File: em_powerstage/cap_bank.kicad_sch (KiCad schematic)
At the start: 20 parts

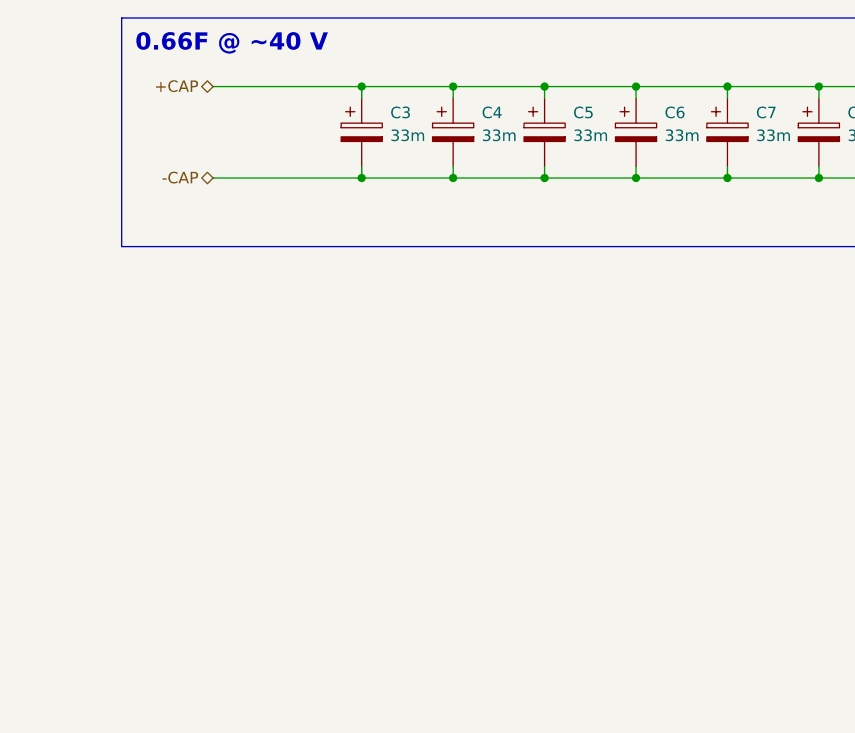
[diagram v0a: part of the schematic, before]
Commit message: updated power stage board
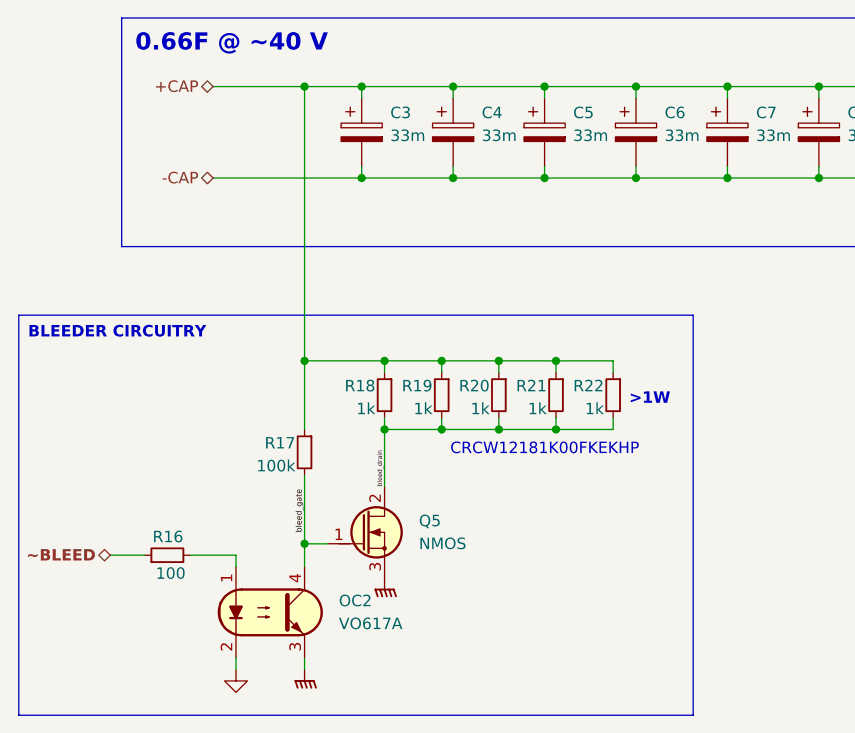
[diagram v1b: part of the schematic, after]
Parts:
- added OC2: VO617A, PCM_Package_DIP_AKL:DIP-4_W7.62mm_LongPads, symbol PCM_Optocoupler_AKL:VO617A
- added Q5: NMOS, Package_TO_SOT_SMD:SOT-23-3, symbol PCM_Transistor_MOSFET_AKL:Q_NMOS-D_Generic_GDS
- added R16: 100, Resistor_SMD:R_0805_2012Metric_Pad1.20x1.40mm_HandSolder, symbol Device:R_Small
- added R17: 100k, Resistor_SMD:R_0805_2012Metric_Pad1.20x1.40mm_HandSolder, symbol Device:R_Small
- added R18, R19, R20, R21, R22: 1k, Resistor_SMD:R_1218_3246Metric_Pad1.22x4.75mm_HandSolder, symbol Device:R_Small
- C10, C11, C12, C13, C14, C15, C16, C17, C18, C19, C20, C21, C22, C3, C4, C5, C6, C7, C8, C9: footprint Capacitor_THT:CP_Radial_D22.0mm_P10.00mm_SnapIn -> HAVENS_Lib:CAPPRD1000W190D3550H8200
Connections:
- net +CAP: now also R17.1, R18.1, R19.1, R20.1, R21.1, R22.1
- new net: OC2.1, R16.2
- new net GND: OC2.2
- new net GNDPWR: OC2.3, Q5.3 (S)
- new net bleed_drain: Q5.2 (D), R18.2, R19.2, R20.2, R21.2, R22.2
- new net bleed_gate: OC2.4, Q5.1 (G), R17.2
- new net ~BLEED: R16.1
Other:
- note added: ">1W"
- note added: "CRCW12181K00FKEKHP"
